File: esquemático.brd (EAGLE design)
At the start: 70.1 x 59.1 mm, 28 parts, among them Q1 MMBT4403LT1SMD, Q3 MMBT4403LT1SMD, U3 AP2210N-4.0TRG1, X1 MKDSN1,5/2-5,08, X2 MKDSN1,5/2-5,08, X3 MKDSN1,5/2-5,08, X4 MKDSN1,5/2-5,08

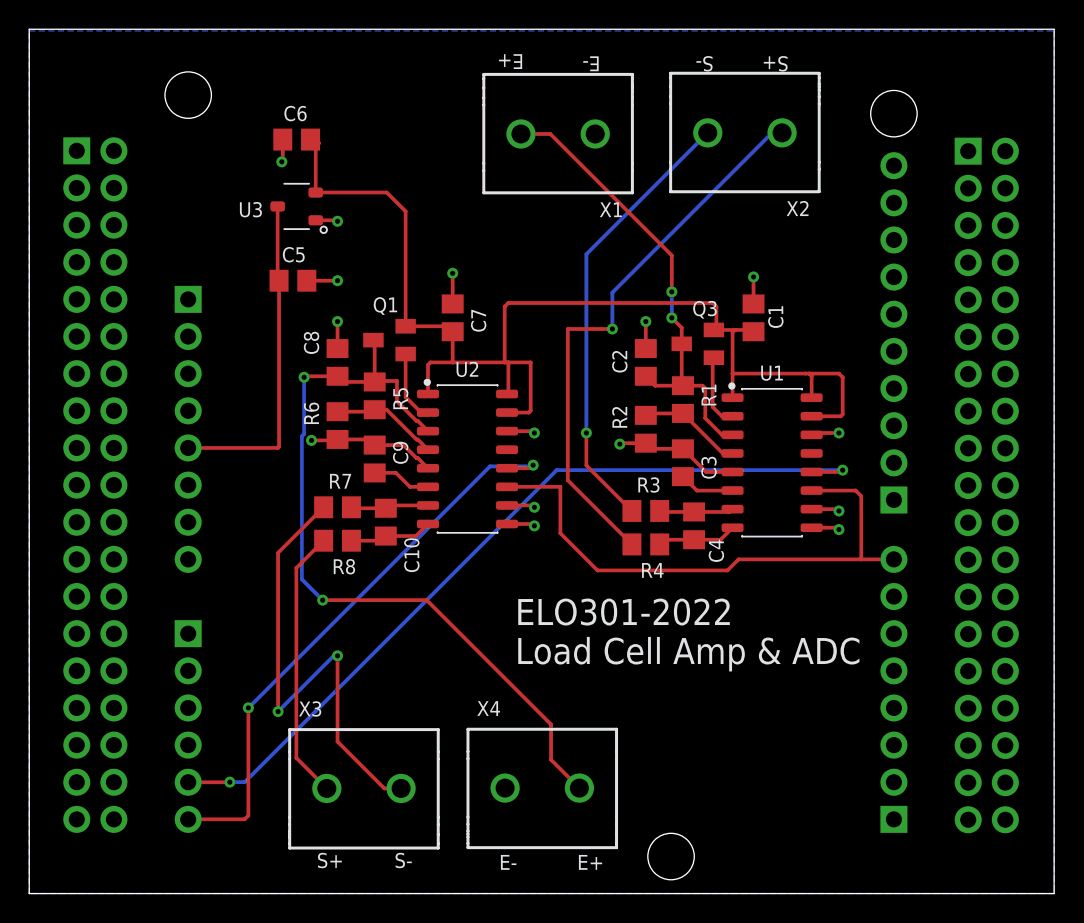
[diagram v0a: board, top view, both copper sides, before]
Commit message: Add files via upload
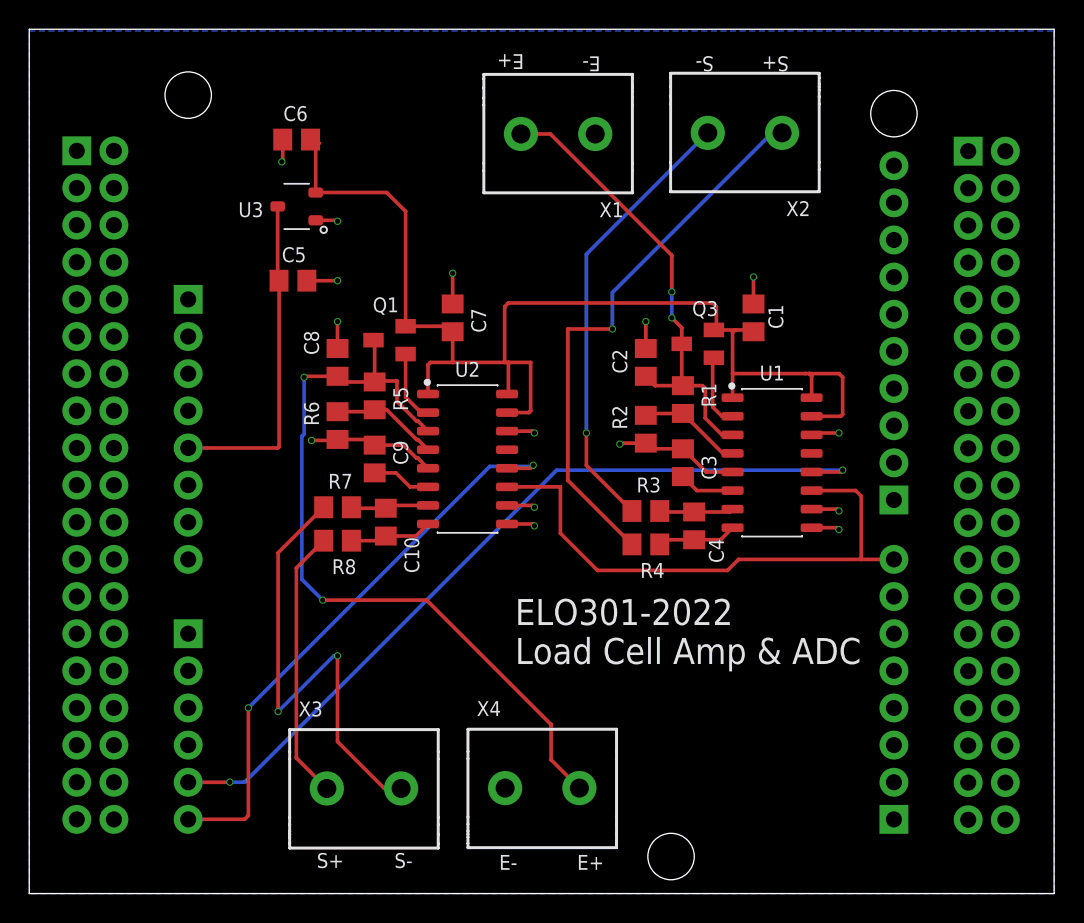
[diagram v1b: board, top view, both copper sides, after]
